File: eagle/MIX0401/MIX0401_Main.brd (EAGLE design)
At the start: 70.8 x 45.7 mm, 30 parts, among them IC1 NJM4580, IC2 NJM4580

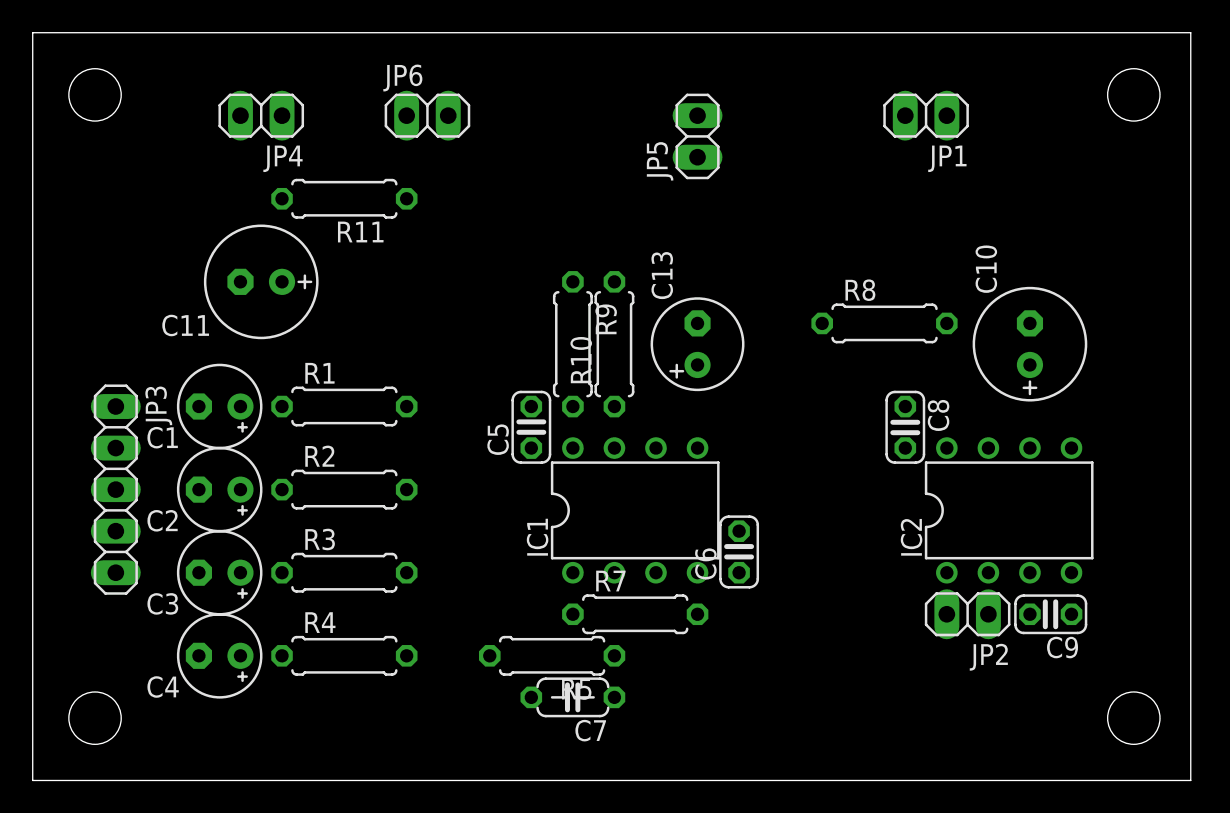
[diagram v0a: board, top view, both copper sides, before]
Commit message: Update: Eagle files
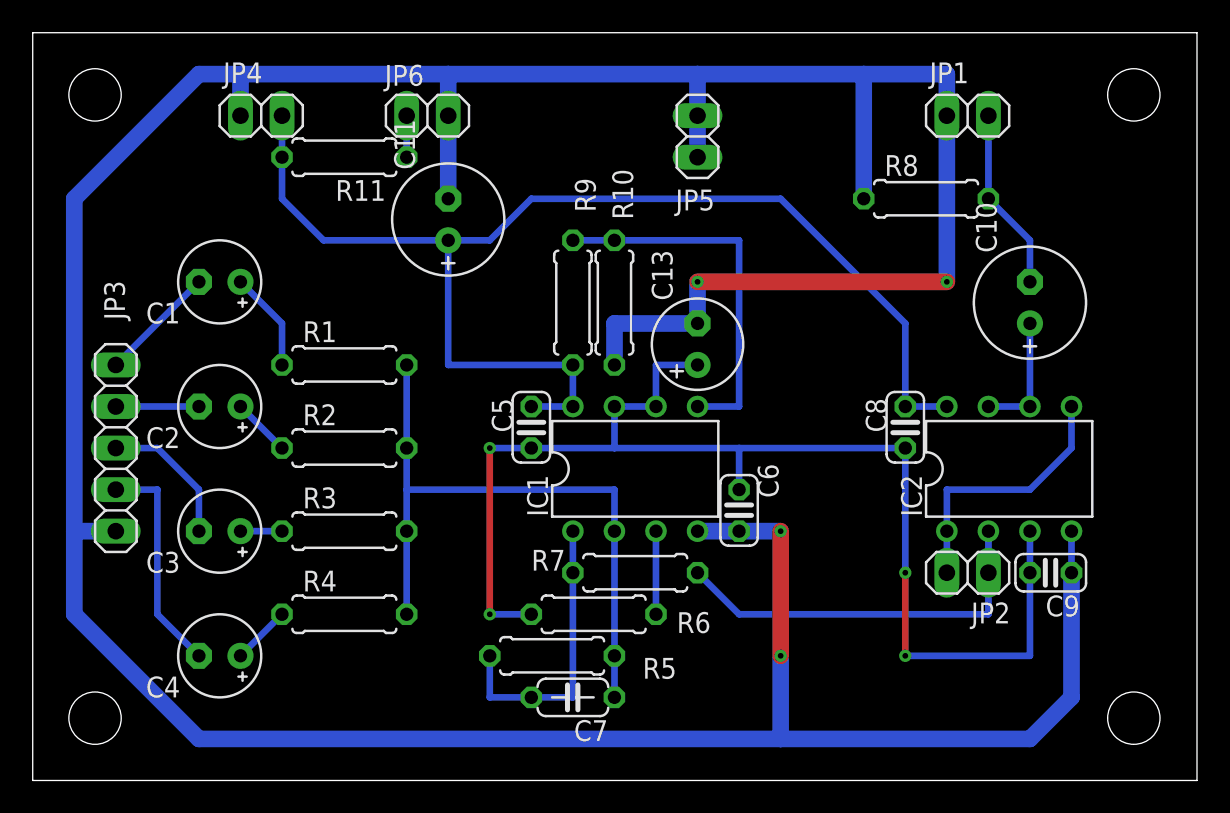
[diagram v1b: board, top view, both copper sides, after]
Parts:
- added R6: 2.2k, rcl:0207/7
- moved C11 12.0 mm to (25.4, 34.3), turned to 90 degrees
- moved R8 8.03 mm to (54.6, 35.6)
- moved C1 7.62 mm to (11.4, 30.5)
- moved C2 5.08 mm to (11.4, 22.9)
- moved C3 2.54 mm to (11.4, 15.2)
- moved C6 2.54 mm to (43.2, 16.5)
- moved R3 2.54 mm to (19.1, 15.2)
- moved R4 2.54 mm to (19.1, 10.2)
- moved C10 2.54 mm to (61.0, 29.2)
- moved C9 2.54 mm to (62.2, 12.7)
- moved IC1 2.54 mm to (36.8, 19.1)
- moved IC2 2.54 mm to (59.7, 19.1)
- moved JP1 2.54 mm to (57.1, 40.6)
- moved JP2 2.54 mm to (57.1, 12.7)
- moved JP3 2.54 mm to (5.08, 20.3)
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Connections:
- new net N$3: IC1.3, R6.2
- net VCC/2: now also R6.1; no longer IC1.3
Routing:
- net GND: track 0.00 -> 238.5 mm, vias 0 -> 4
- net VCC/2: track 0.00 -> 78.7 mm, vias 0 -> 4
- net VCC: track 0.00 -> 76.4 mm
- net N$1: track 0.00 -> 40.6 mm
- net N$4: track 0.00 -> 23.9 mm
- net N$11: track 0.00 -> 22.9 mm
- net N$6: track 0.00 -> 17.8 mm
- net N$13: track 0.00 -> 16.3 mm
- net N$16: track 0.00 -> 13.8 mm
- net N$10: track 0.00 -> 11.2 mm
- net N$15: track 0.00 -> 8.67 mm
- net N$12: track 0.00 -> 7.62 mm
- net N$2: track 0.00 -> 7.18 mm
- net N$5: track 0.00 -> 6.13 mm
- net N$3: track 0.00 -> 5.08 mm
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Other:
- board size 70.8 x 45.7 mm -> 71.2 x 45.7 mm
- board text added: "MIX0401"
- board text added: "http://dad8893.blogspot.jp/"
